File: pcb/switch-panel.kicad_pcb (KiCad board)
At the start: 2 copper layers, 73.3 x 35.4 mm, 58 parts, among them J1 USB_C_Receptacle_USB2.0_16P, J2 Conn_ARM_SWD_TagConnect_TC203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, Q1 AO3400A, Q2 AO3400A, Q3 AO3400A, Q4 AO3400A, Q5 AO3400A, Q6 AO3400A, Q7 AO3400A, Q8 AO3400A, Q9 AO3400A, SW1 SW_Push, SW2 SW_Push, SW3 SW_Push, U1 AMS1117-3.3, U2 SSD1306, U3 STM32F103C8Tx, U4 SRV05-4, Y1 16MHz

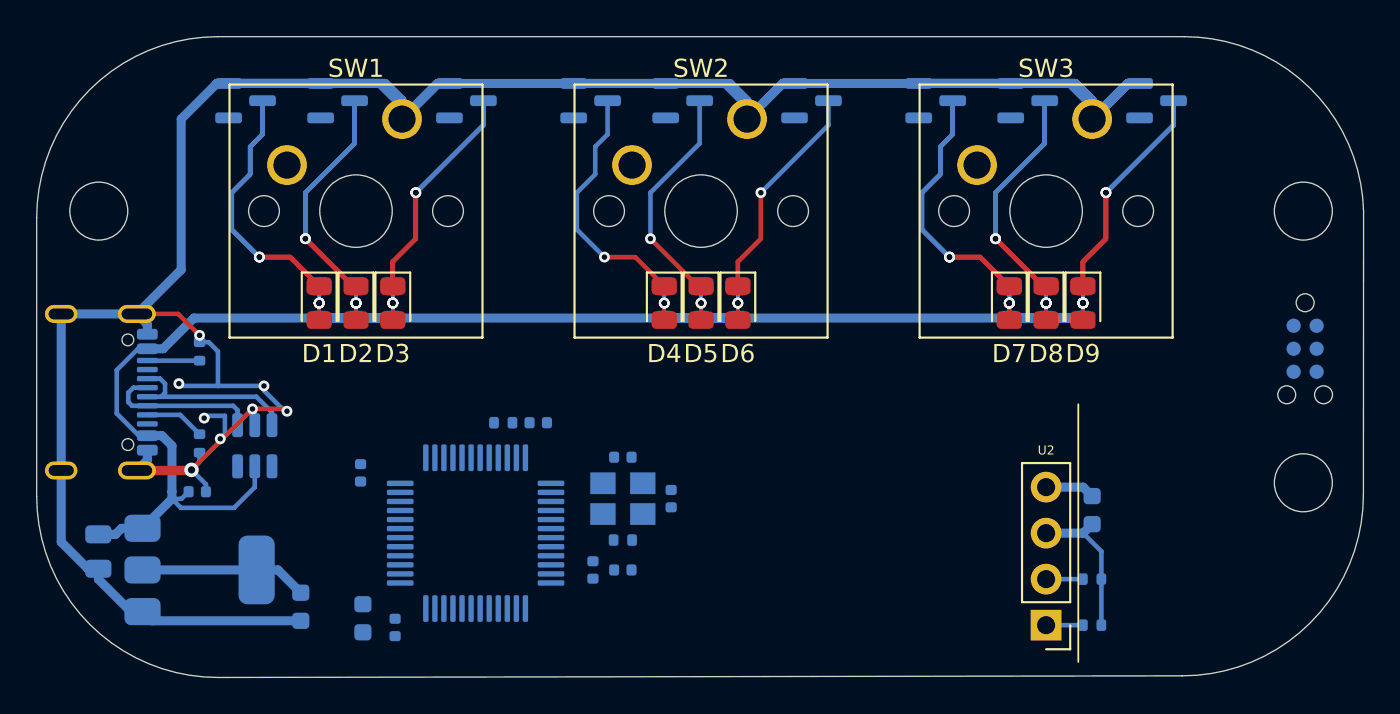
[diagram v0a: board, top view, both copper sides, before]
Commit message: Final routing and production
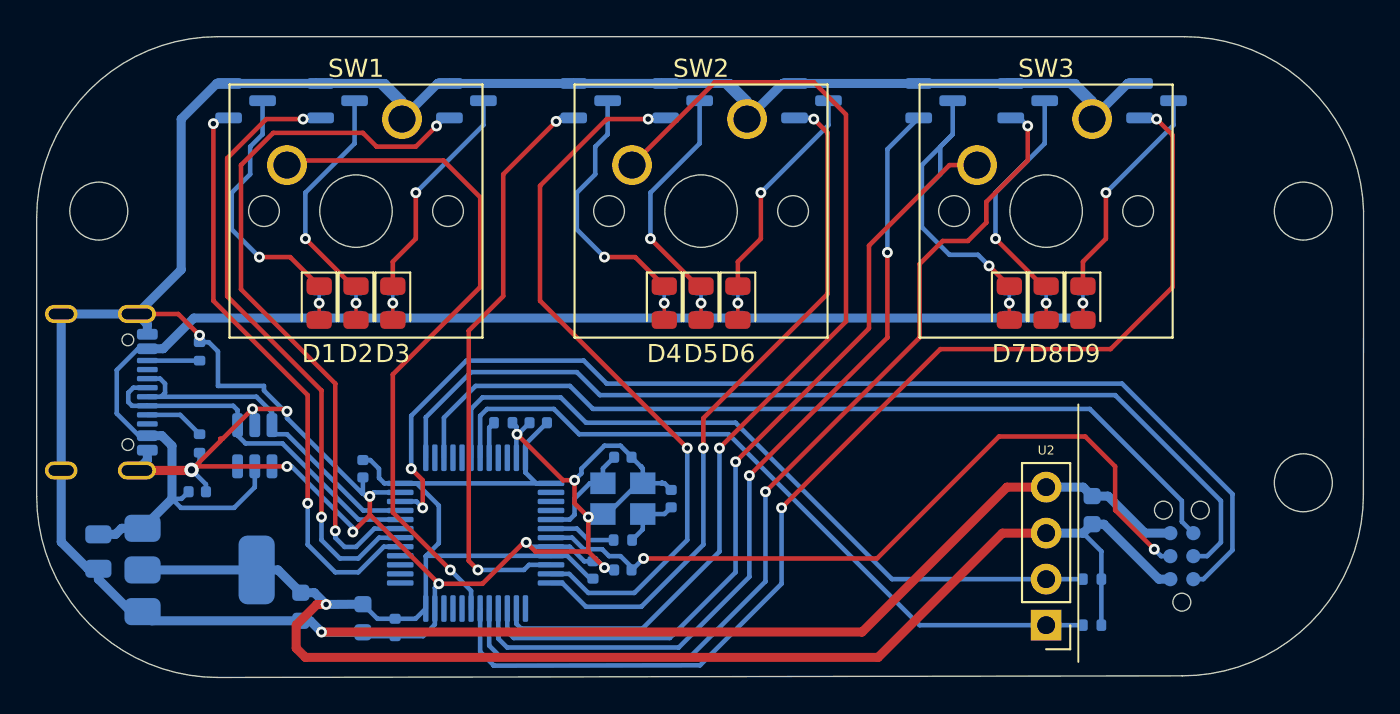
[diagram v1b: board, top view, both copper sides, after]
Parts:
- moved J2 13.3 mm to (121.8, 95.2), turned to 90 degrees
- moved C4 0.26 mm to (76.6, 90.4)
- turned C10 to 180 degrees
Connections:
- U3 pad 13: /BTN1 -> unconnected-(U3-PA3-Pad13)
- U3 pad 19: unconnected-(U3-PB1-Pad19) -> /BTN1
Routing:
- net +3V3: track 17.5 -> 113.2 mm, vias 0 -> 1
- net /LEDB3: track 0.00 -> 62.7 mm, vias 0 -> 2
- net /SWDIO: track 0.00 -> 62.3 mm, vias 0 -> 2
- net /BTN2: track 0.00 -> 55.4 mm, vias 0 -> 1
- net /SWCLK: track 0.00 -> 54.2 mm
- net /LEDG3: track 0.00 -> 52.4 mm, vias 0 -> 2
- net /SWO: track 0.00 -> 48.4 mm
- net /LEDR3: track 0.00 -> 46.6 mm, vias 0 -> 2
- net /BTN3: track 0.00 -> 44.4 mm, vias 0 -> 1
- net /RST: track 0.00 -> 42.2 mm, vias 0 -> 2
- net VBUS: track 116.6 -> 76.0 mm
- net /LEDG2: track 0.00 -> 40.6 mm, vias 0 -> 2
- net /LEDB1: track 0.00 -> 40.2 mm, vias 0 -> 2
- net /SCL: track 2.03 -> 40.9 mm
- net /SDA: track 2.03 -> 40.7 mm
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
